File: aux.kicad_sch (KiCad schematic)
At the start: 15 parts, among them J85 USB_C_Receptacle_USB2.0_16P, J86 Conn_01x02_Pin, Q81 Si2301CDS, Q82 AO3400A, U85 DAC80508xRTE

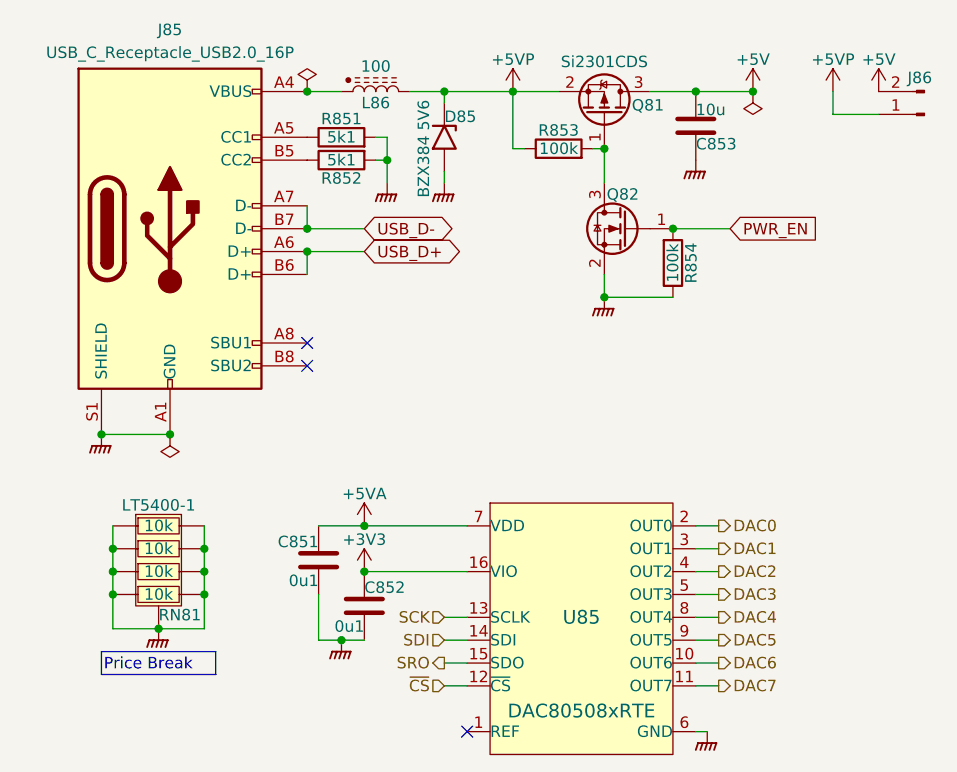
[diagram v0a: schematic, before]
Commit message: Everything assigned except for wierd shit.
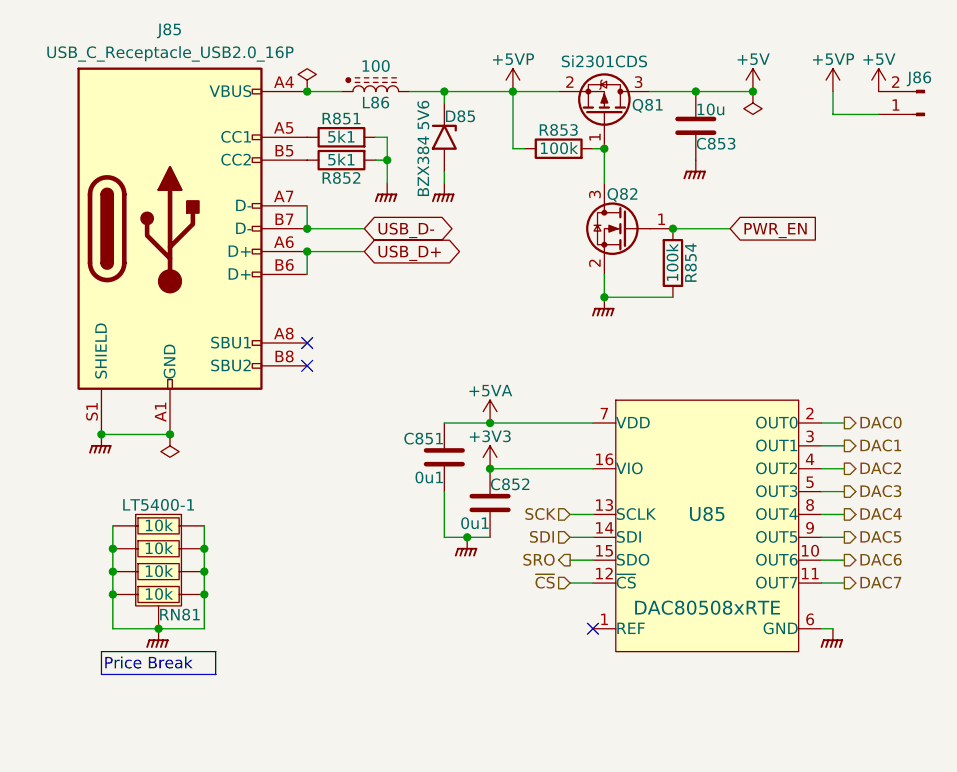
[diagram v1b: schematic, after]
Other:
- moved on the sheet: C851, C852, U85
